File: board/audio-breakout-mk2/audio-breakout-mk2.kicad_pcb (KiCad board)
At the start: 2 copper layers, 24 x 21 mm, 2 parts, among them J1 Conn_01x06_Socket

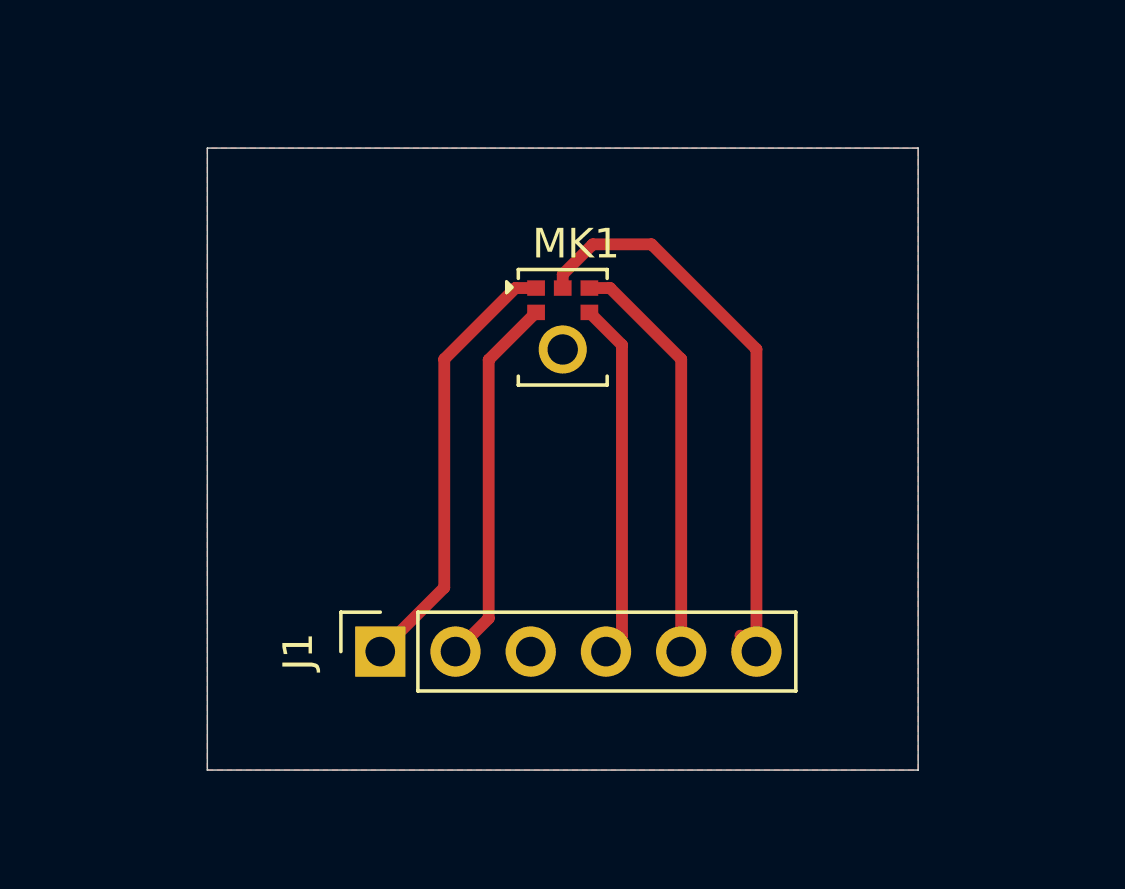
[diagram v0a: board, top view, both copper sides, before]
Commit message: audio board mk2
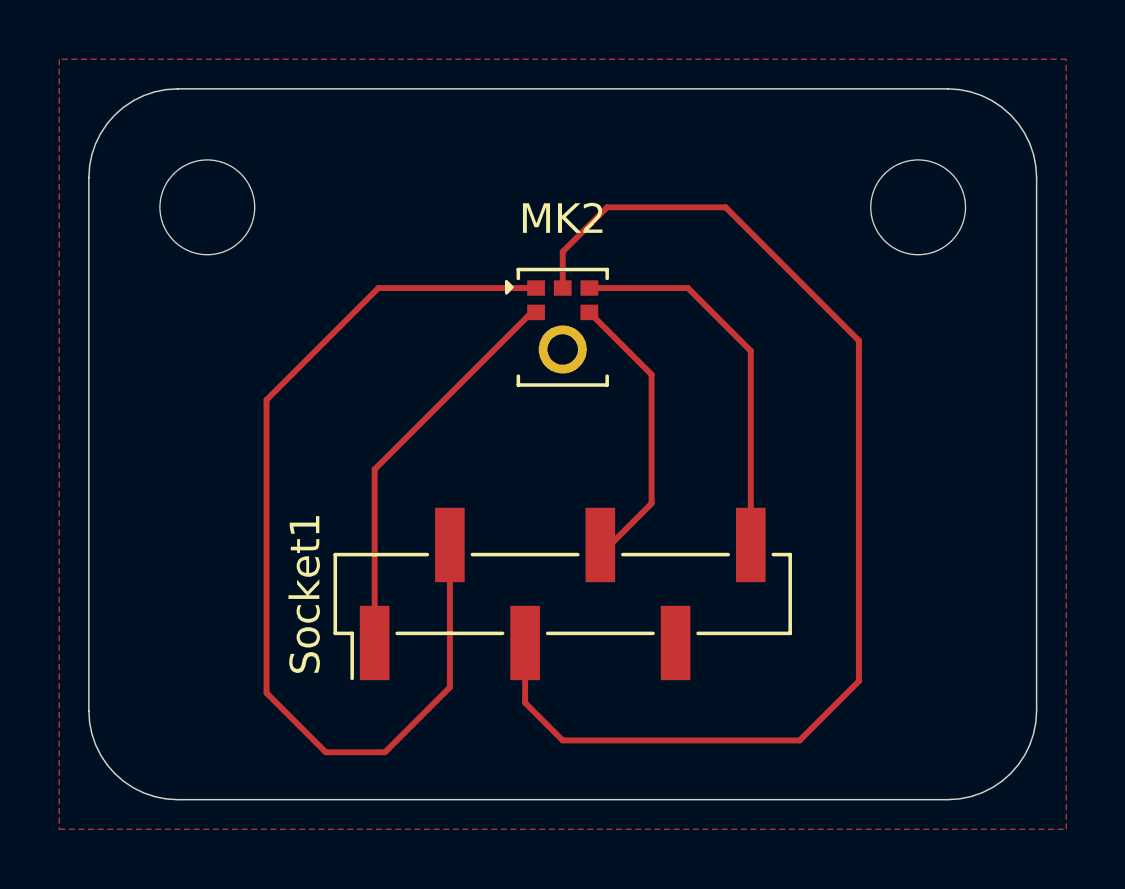
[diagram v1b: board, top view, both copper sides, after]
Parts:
- added REF**: MountingHole_3.2mm_M3, MountingHole:MountingHole_3.2mm_M3, F.Cu at (130.0, 70.0)
- added REF**: MountingHole_3.2mm_M3, MountingHole:MountingHole_3.2mm_M3, F.Cu at (154.0, 70.0)
- Socket1: renamed from J1; footprint Connector_PinSocket_2.54mm:PinSocket_1x06_P2.54mm_Vertical -> Connector_PinHeader_2.54mm:PinHeader_1x06_P2.54mm_Vertical_SMD_Pin1Left
- moved Socket1 6.46 mm to (142.0, 83.1)
- renumbered MK1 to MK2
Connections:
- MK2 pad 1: Net-(J1-Pin_1) -> Net-(MK1-WS)
- MK2 pad 2: Net-(J1-Pin_2) -> Net-(MK1-LR)
- MK2 pad 5: Net-(J1-Pin_5) -> Net-(MK1-VDD)
- MK2 pad 6: Net-(J1-Pin_6) -> Net-(MK1-SD)
- Socket1 pad 1: Net-(J1-Pin_1) -> Net-(MK1-LR)
- Socket1 pad 2: Net-(J1-Pin_2) -> Net-(MK1-WS)
- Socket1 pad 3: GND -> Net-(MK1-SD)
- Socket1 pad 5: Net-(J1-Pin_5) -> GND
- Socket1 pad 6: Net-(J1-Pin_6) -> Net-(MK1-VDD)
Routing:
- net Net-(MK1-SD): track 0.00 -> 39.9 mm
- net Net-(MK1-WS): track 0.00 -> 33.3 mm
- net Net-(J1-Pin_6): track 19.9 -> 0.00 mm
- net Net-(J1-Pin_1): track 14.9 -> 0.00 mm
- net Net-(J1-Pin_5): track 14.0 -> 0.00 mm
- net Net-(MK1-LR): track 0.00 -> 13.5 mm
- net Net-(MK1-VDD): track 0.00 -> 12.9 mm
- net Net-(J1-Pin_2): track 12.6 -> 0.00 mm
- net Net-(MK1-SCK): track 12.1 -> 9.63 mm
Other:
- board size 24 x 21 mm -> 32 x 24 mm
